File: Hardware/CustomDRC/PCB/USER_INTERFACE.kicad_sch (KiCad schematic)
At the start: 35 parts, among them J501 Conn_01x05, J504 Conn_01x05, Q501 AO3401A, Q502 AO3400A, U501 ESD224DQA, U502 ESD224DQA

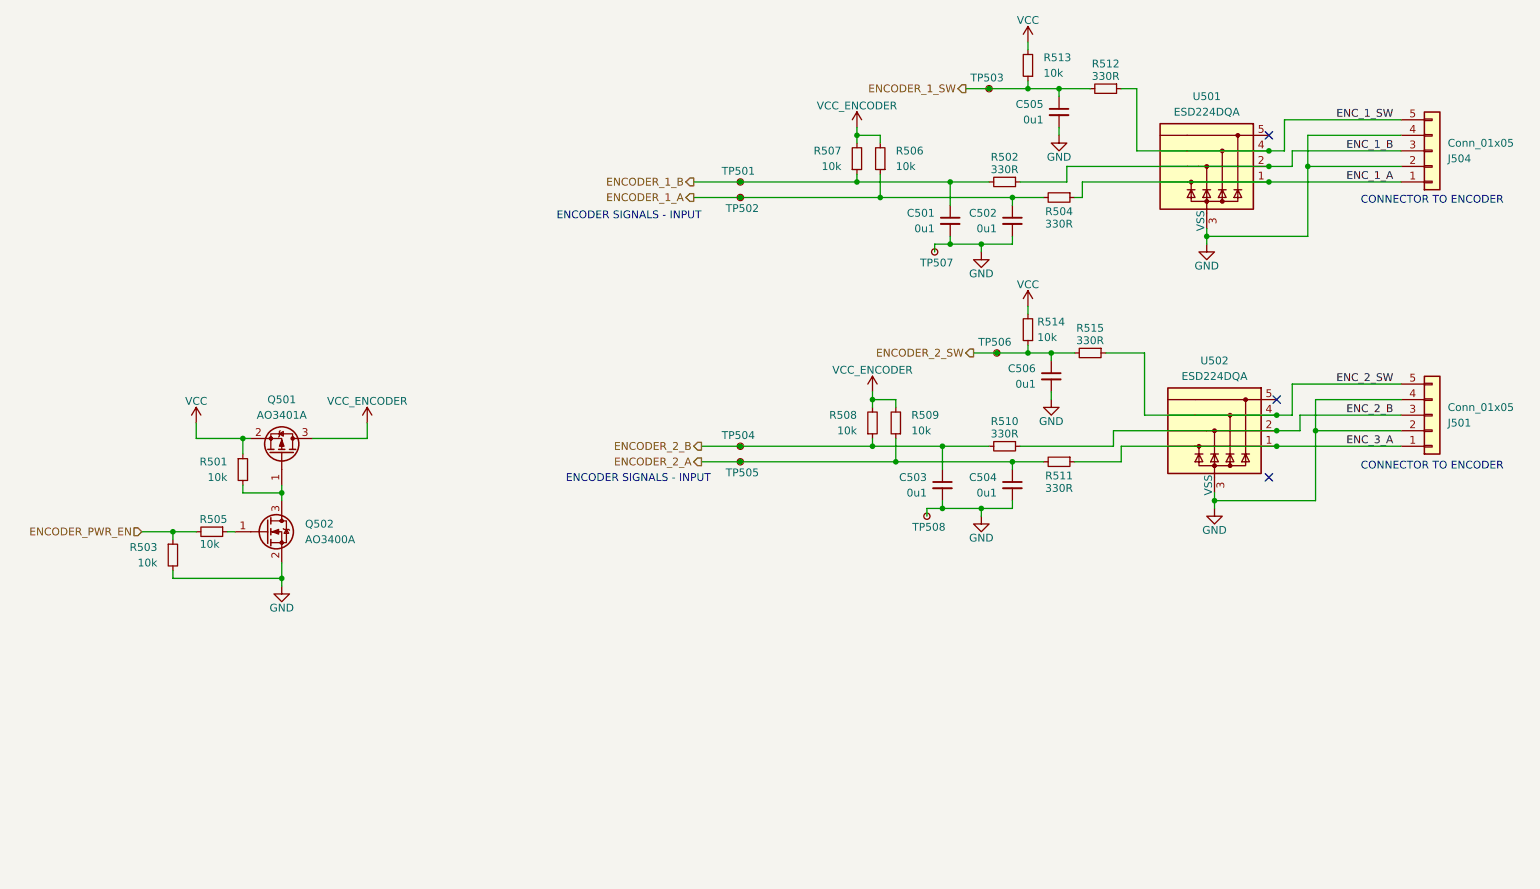
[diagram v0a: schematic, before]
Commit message: Update - finished schematic for revision A
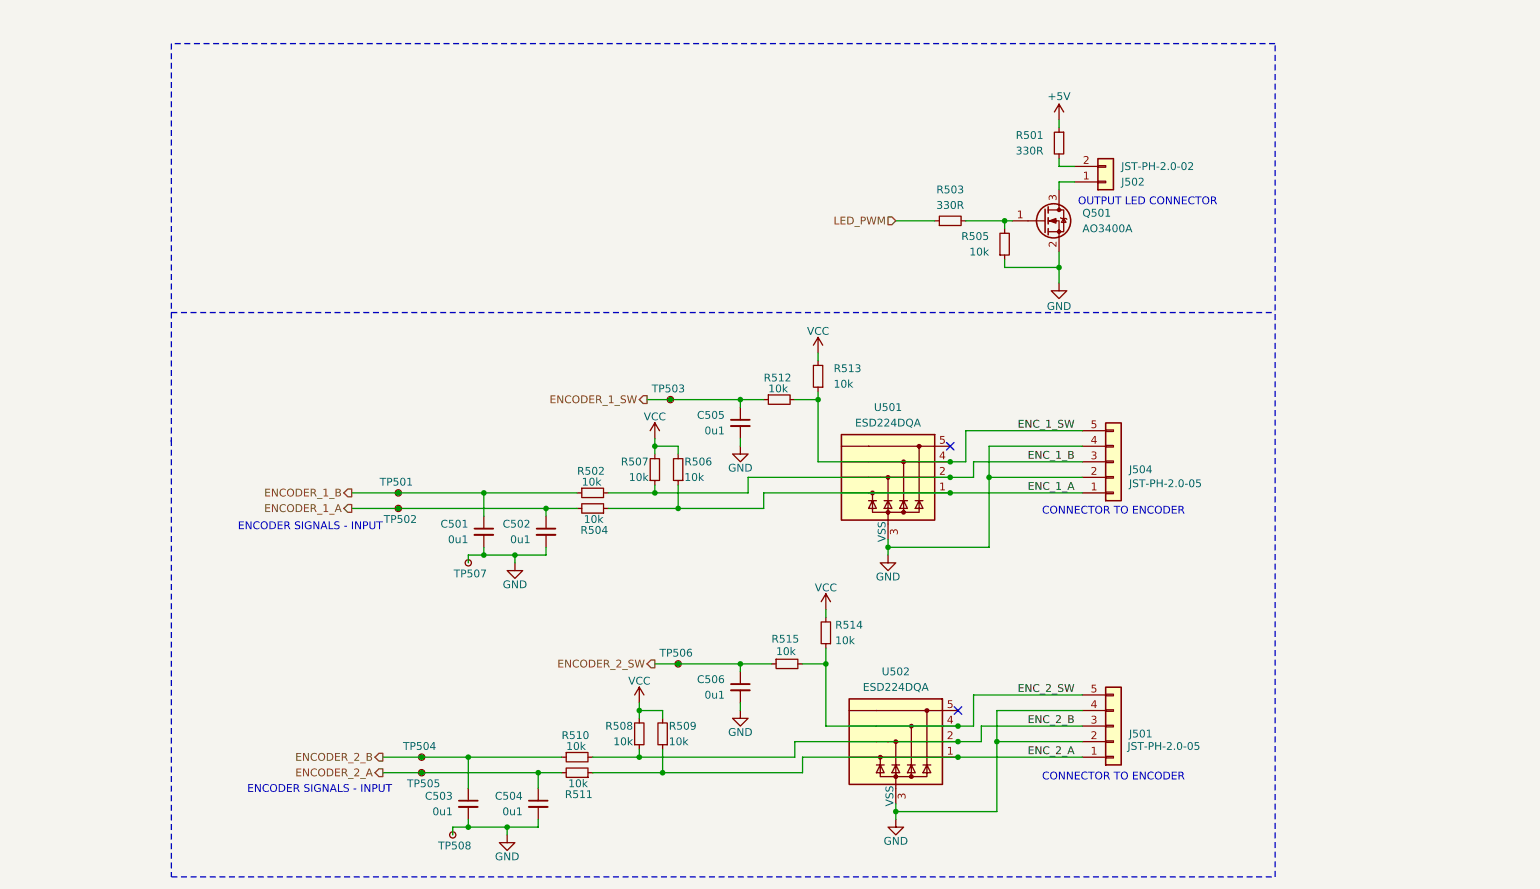
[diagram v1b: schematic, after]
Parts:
- removed Q501: AO3401A, Package_TO_SOT_SMD:SOT-23, symbol Transistor_FET:AO3401A
- removed Q502: AO3400A, Package_TO_SOT_SMD:SOT-23, symbol Transistor_FET:AO3400A
- added J502: JST-PH-2.0-02, Connector_JST:JST_PH_B2B-PH-K_1x02_P2.00mm_Vertical, symbol Connector_Generic:Conn_01x02
- added Q501: AO3400A, Package_TO_SOT_SMD:SOT-23, symbol Transistor_FET:AO3400A
- C501, C502, C503, C504, C505, C506: LCSC (none) -> C14663; MPN (none) -> CC0603KRX7R9BB104; Manufacturer (none) -> YAGEO
- J501, J504: value Conn_01x05 -> JST-PH-2.0-05; LCSC (none) -> C157993; MPN (none) -> B5B-PH-K-S(LF)(SN); Manufacturer (none) -> JST
- R501, R503: value 10k -> 330R; LCSC (none) -> C23138; MPN (none) -> 0603WAF3300T5E; Manufacturer (none) -> UNI-ROYAL(Uniroyal Elec)
- R502, R504, R510, R511, R512, R515: value 330R -> 10k; LCSC (none) -> C25804; MPN (none) -> 0603WAF1002T5E; Manufacturer (none) -> UNI-ROYAL(Uniroyal Elec)
- R505, R506, R507, R508, R509, R513, R514: LCSC (none) -> C25804; MPN (none) -> 0603WAF1002T5E; Manufacturer (none) -> UNI-ROYAL(Uniroyal Elec)
- TP508: footprint TestPoint:TestPoint_Pad_D1.5mm -> TestPoint:TestPoint_Keystone_5000-5004_Miniature; LCSC (none) -> C5199801; MPN (none) -> RH-5001; Manufacturer (none) -> ronghe; now in the parts list
- U501, U502: LCSC (none) -> C5199157; MPN (none) -> RClAMP3324P-ES; Manufacturer (none) -> ElecSuper
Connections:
- net VCC_ENCODER is gone; now on net VCC: R506.2, R507.2, R508.2, R509.2
- net ENCODER_1_A: no longer R506.1
- net ENCODER_1_B: now also R502.1; no longer R502.2, R507.1
- net ENCODER_1_SW: now also R512.1; no longer R512.2, R513.1
- net ENCODER_2_A: no longer R509.1
- net ENCODER_2_B: now also R510.1; no longer R508.1, R510.2
- net ENCODER_2_SW: now also R515.1; no longer R514.1, R515.2
- net ENC_1_A: now also R506.1
- net ENC_1_B: now also R502.2, R507.1; no longer R502.1
- net ENC_1_SW: now also R512.2, R513.1; no longer R512.1
- net ENC_2_B: now also R508.1, R510.2; no longer R510.1
- net ENC_2_SW: now also R514.1, R515.2; no longer R515.1
- net GND: now also R505.1, Q501.2 (S); no longer R503.2
- net VCC: no longer R501.1
- net at R501.2: now also J502.2 (Pin_2)
- net ENCODER_PWR_EN: no longer names the net of R505.2
- net ENCODER_PWR_EN: now also R503.2, Q501.1 (G); no longer R503.1
- net ENC_3_A renamed ENC_2_A
- net ENC_2_A: now also R509.1
- new net: J502.1 (Pin_1), Q501.3 (D)
- new net +5V: R501.1
- new net LED_PWM: R503.1
- no-connect marks 3 -> 2
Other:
- note added: "OUTPUT LED CONNECTOR"
- company: (none) -> JS HW
- title: (none) -> CDRC - Custom DRC for Audison AC Link
- moved on the sheet: C501, C502, C503, C504, C505, C506, J501, J504, R506, R507, R508, R509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
